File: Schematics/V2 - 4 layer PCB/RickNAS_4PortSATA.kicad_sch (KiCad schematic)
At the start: 29 parts, among them J1 2227595-1, J10 10076579-002C-TRLF, J6 POWER, J7 10076579-002C-TRLF, J8 10076579-002C-TRLF, J9 10076579-002C-TRLF, U1 CH32V003FxPx

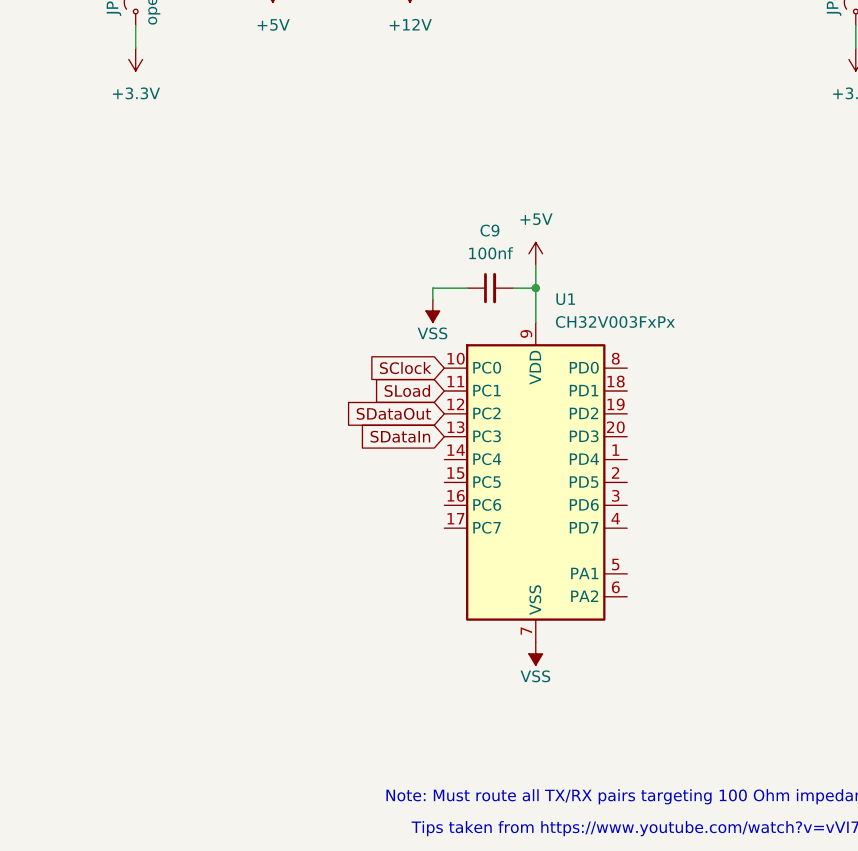
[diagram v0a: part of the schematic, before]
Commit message: Progress on V2
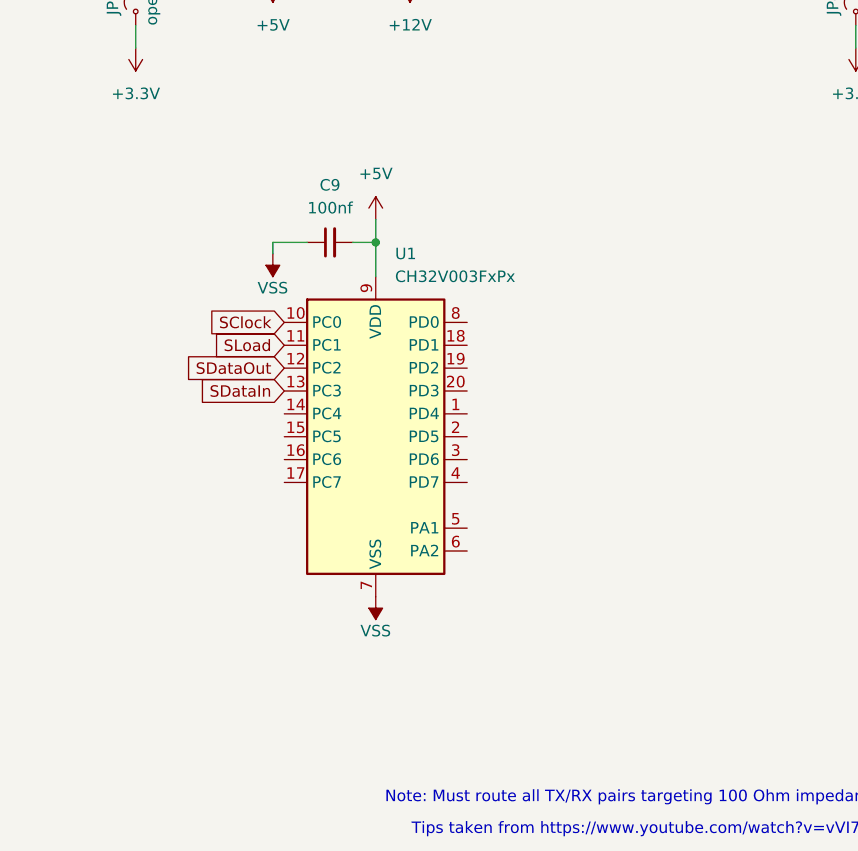
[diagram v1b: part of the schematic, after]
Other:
- moved on the sheet: C9, U1
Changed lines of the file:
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@@
 	)
 	(junction
-		(at 209.55 114.3)
+		(at 191.77 109.22)
 		(diameter 0)
 		(color 0 0 0 0)
@@
 	(wire
 		(pts
-			(xy 209.55 111.76) (xy 209.55 114.3)
+			(xy 191.77 106.68) (xy 191.77 109.22)
 		)
 		(stroke
@@
 	(wire
 		(pts
-			(xy 198.12 115.57) (xy 198.12 114.3)
+			(xy 180.34 110.49) (xy 180.34 109.22)
 		)
 		(stroke
@@
 	(wire
 		(pts
-			(xy 207.01 114.3) (xy 209.55 114.3)
+			(xy 189.23 109.22) (xy 191.77 109.22)
 		)
 		(stroke
@@
 	(wire
 		(pts
-			(xy 209.55 114.3) (xy 209.55 118.11)
+			(xy 191.77 109.22) (xy 191.77 113.03)
 		)
 		(stroke
@@
 	(wire
 		(pts
-			(xy 198.12 114.3) (xy 201.93 114.3)
+			(xy 180.34 109.22) (xy 184.15 109.22)
 		)
 		(stroke
@@
 	(global_label "SDataOut"
 		(shape input)
-		(at 199.39 128.27 180)
+		(at 181.61 123.19 180)
 		(fields_autoplaced yes)
 		(effects
@@
 		)
 		(property "Intersheetrefs" "${INTERSHEET_REFS}"
-			(at 187.6964 128.27 0)
+			(at 169.9164 123.19 0)
 			(effects
 				(font
@@
 	(global_label "SDataIn"
 		(shape input)
-		(at 199.39 130.81 180)
+		(at 181.61 125.73 180)
 		(fields_autoplaced yes)
 		(effects
@@
 		)
 		(property "Intersheetrefs" "${INTERSHEET_REFS}"
-			(at 189.1478 130.81 0)
+			(at 171.3678 125.73 0)
 			(effects
 				(font
@@
 	(global_label "SClock"
 		(shape input)
-		(at 199.39 123.19 180)
+		(at 181.61 118.11 180)
 		(fields_autoplaced yes)
 		(effects
@@
 		)
 		(property "Intersheetrefs" "${INTERSHEET_REFS}"
-			(at 189.9944 123.19 0)
+			(at 172.2144 118.11 0)
 			(effects
 				(font
@@
 	(global_label "SLoad"
 		(shape input)
-		(at 199.39 125.73 180)
+		(at 181.61 120.65 180)
 		(fields_autoplaced yes)
 		(effects
@@
 		)
 		(property "Intersheetrefs" "${INTERSHEET_REFS}"
-			(at 190.7202 125.73 0)
+			(at 172.9402 120.65 0)
 			(effects
 				(font
@@
 	(symbol
 		(lib_id "power:VSS")
-		(at 209.55 153.67 180)
+		(at 191.77 148.59 180)
 		(unit 1)
 		(exclude_from_sim no)
@@
 		(dnp no)
 		(property "Reference" "#PWR095"
-			(at 209.55 149.86 0)
+			(at 191.77 144.78 0)
 			(effects
 				(font
@@
 		)
 		(property "Value" "VSS"
-			(at 209.55 157.48 0)
+			(at 191.77 152.4 0)
 			(effects
 				(font
@@
 		)
 		(property "Footprint" ""
-			(at 209.55 153.67 0)
+			(at 191.77 148.59 0)
 			(effects
 				(font
@@
 		)
 		(property "Datasheet" ""
-			(at 209.55 153.67 0)
+			(at 191.77 148.59 0)
 			(effects
 				(font
@@
 		)
 		(property "Description" "Power symbol creates a global label with name \"VSS\""
-			(at 209.55 153.67 0)
+			(at 191.77 148.59 0)
 			(effects
 				(font
@@
 	(symbol
 		(lib_id "power:+5V")
-		(at 209.55 111.76 0)
+		(at 191.77 106.68 0)
 		(unit 1)
 		(exclude_from_sim no)
@@
 		(fields_autoplaced yes)
 		(property "Reference" "#PWR093"
-			(at 209.55 115.57 0)
+			(at 191.77 110.49 0)
 			(effects
 				(font
@@
 		)
 		(property "Value" "+5V"
-			(at 209.55 106.68 0)
+			(at 191.77 101.6 0)
 			(effects
 				(font
@@
 		)
 		(property "Footprint" ""
-			(at 209.55 111.76 0)
+			(at 191.77 106.68 0)
 			(effects
 				(font
@@
 		)
 		(property "Datasheet" ""
-			(at 209.55 111.76 0)
+			(at 191.77 106.68 0)
 			(effects
 				(font
@@
 		)
 		(property "Description" ""
-			(at 209.55 111.76 0)
+			(at 191.77 106.68 0)
 			(effects
 				(font
@@
 	(symbol
 		(lib_id "MCU_WCH_CH32V0:CH32V003FxPx")
-		(at 209.55 135.89 0)
+		(at 191.77 130.81 0)
 		(unit 1)
 		(exclude_from_sim no)
@@
 		(fields_autoplaced yes)
 		(property "Reference" "U1"
-			(at 211.6933 115.57 0)
+			(at 193.9133 110.49 0)
 			(effects
 				(font
@@
 		)
 		(property "Value" "CH32V003FxPx"
-			(at 211.6933 118.11 0)
+			(at 193.9133 113.03 0)
 			(effects
 				(font
@@
 		)
 		(property "Footprint" "Package_SO:TSSOP-20_4.4x6.5mm_P0.65mm"
-			(at 208.28 135.89 0)
+			(at 190.5 130.81 0)
 			(effects
 				(font
@@
 		)
 		(property "Datasheet" "https://www.wch-ic.com/products/CH32V003.html"
-			(at 208.28 135.89 0)
+			(at 190.5 130.81 0)
 			(effects
 				(font
@@
 		)
 		(property "Description" "CH32V003 series are industrial-grade general-purpose microcontrollers designed based on 32-bit RISC-V instruction set and architecture. It adopts QingKe V2A core, RV32EC instruction set, and supports 2 levels of interrupt nesting. The series are mounted with rich peripheral interfaces and function modules. Its internal organizational structure meets the low-cost and low-power embedded application scenarios."
-			(at 209.55 135.89 0)
+			(at 191.77 130.81 0)
 			(effects
 				(font
@@
 	(symbol
 		(lib_id "power:VSS")
-		(at 198.12 115.57 180)
+		(at 180.34 110.49 180)
 		(unit 1)
 		(exclude_from_sim no)
@@
 		(dnp no)
 		(property "Reference" "#PWR094"
-			(at 198.12 111.76 0)
+			(at 180.34 106.68 0)
 			(effects
 				(font
@@
 		)
 		(property "Value" "VSS"
-			(at 198.12 119.38 0)
+			(at 180.34 114.3 0)
 			(effects
 				(font
@@
 		)
 		(property "Footprint" ""
-			(at 198.12 115.57 0)
+			(at 180.34 110.49 0)
 			(effects
 				(font
@@
 		)
 		(property "Datasheet" ""
-			(at 198.12 115.57 0)
+			(at 180.34 110.49 0)
 			(effects
 				(font
@@
 		)
 		(property "Description" "Power symbol creates a global label with name \"VSS\""
-			(at 198.12 115.57 0)
+			(at 180.34 110.49 0)
 			(effects
 				(font
@@
 	(symbol
 		(lib_id "Device:C_Small")
-		(at 204.47 114.3 90)
+		(at 186.69 109.22 90)
 		(unit 1)
 		(exclude_from_sim no)
@@
 		(fields_autoplaced yes)
 		(property "Reference" "C9"
-			(at 204.4763 107.95 90)
+			(at 186.6963 102.87 90)
 			(effects
 				(font
@@
 		)
 		(property "Value" "100nf"
-			(at 204.4763 110.49 90)
+			(at 186.6963 105.41 90)
 			(effects
 				(font
@@
 		)
 		(property "Footprint" "Capacitor_SMD:C_0805_2012Metric"
-			(at 204.47 114.3 0)
+			(at 186.69 109.22 0)
 			(effects
 				(font
@@
 		)
 		(property "Datasheet" "~"
-			(at 204.47 114.3 0)
+			(at 186.69 109.22 0)
 			(effects
 				(font
@@
 		)
 		(property "Description" "Unpolarized capacitor, small symbol"
-			(at 204.47 114.3 0)
+			(at 186.69 109.22 0)
 			(effects
 				(font
